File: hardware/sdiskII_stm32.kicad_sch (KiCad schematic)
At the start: 17 parts, among them J1 PWR, J2 APPLE_SDISKII, J3 Conn_01x06, J4 UART, J5 Conn_01x04, J6 STLINK, U2 MicroSD_SDIO, U8 DM-OLED096-636

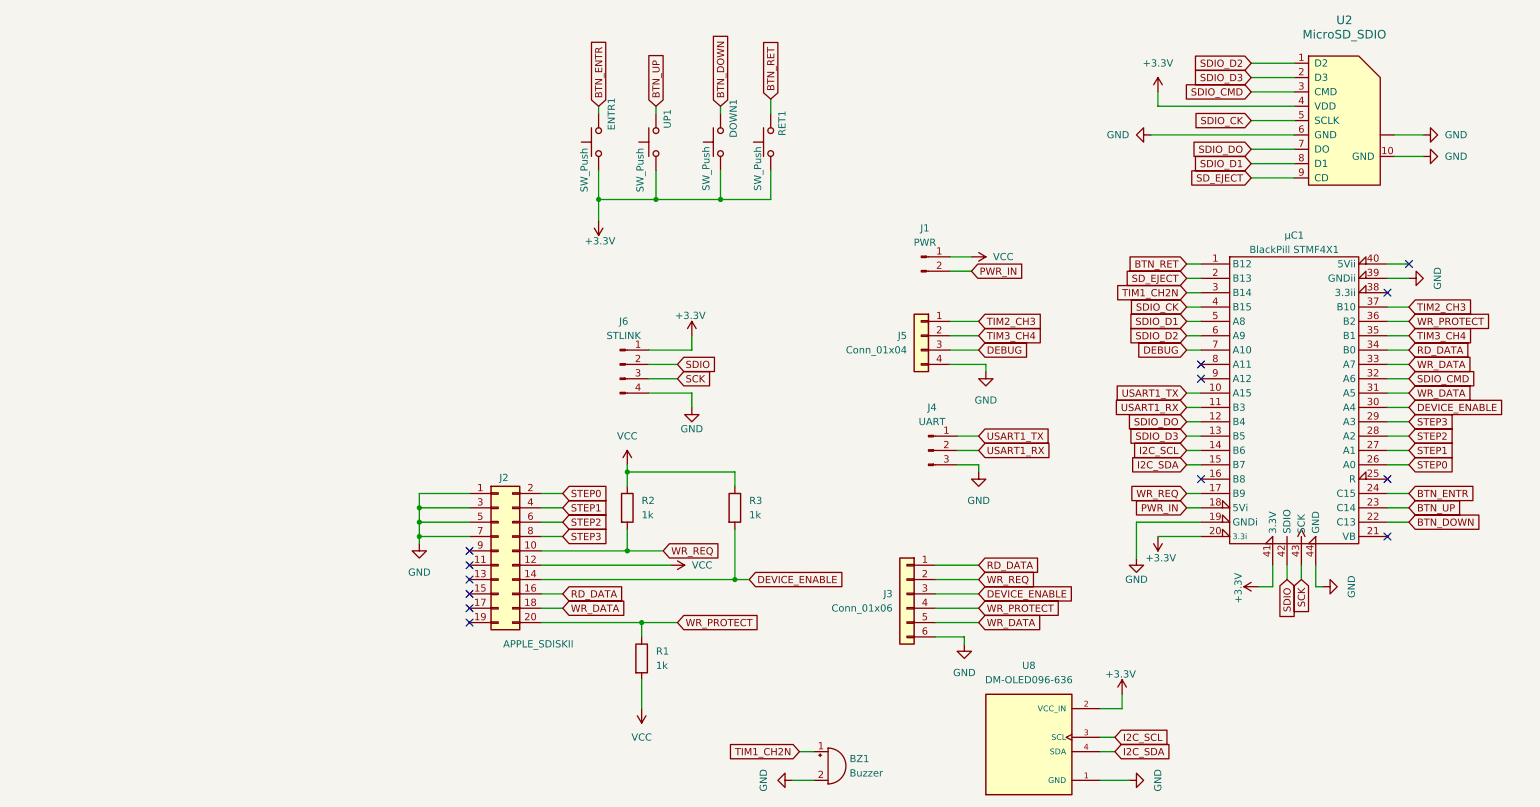
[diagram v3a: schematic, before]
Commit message: v0.79 Smartport HD working
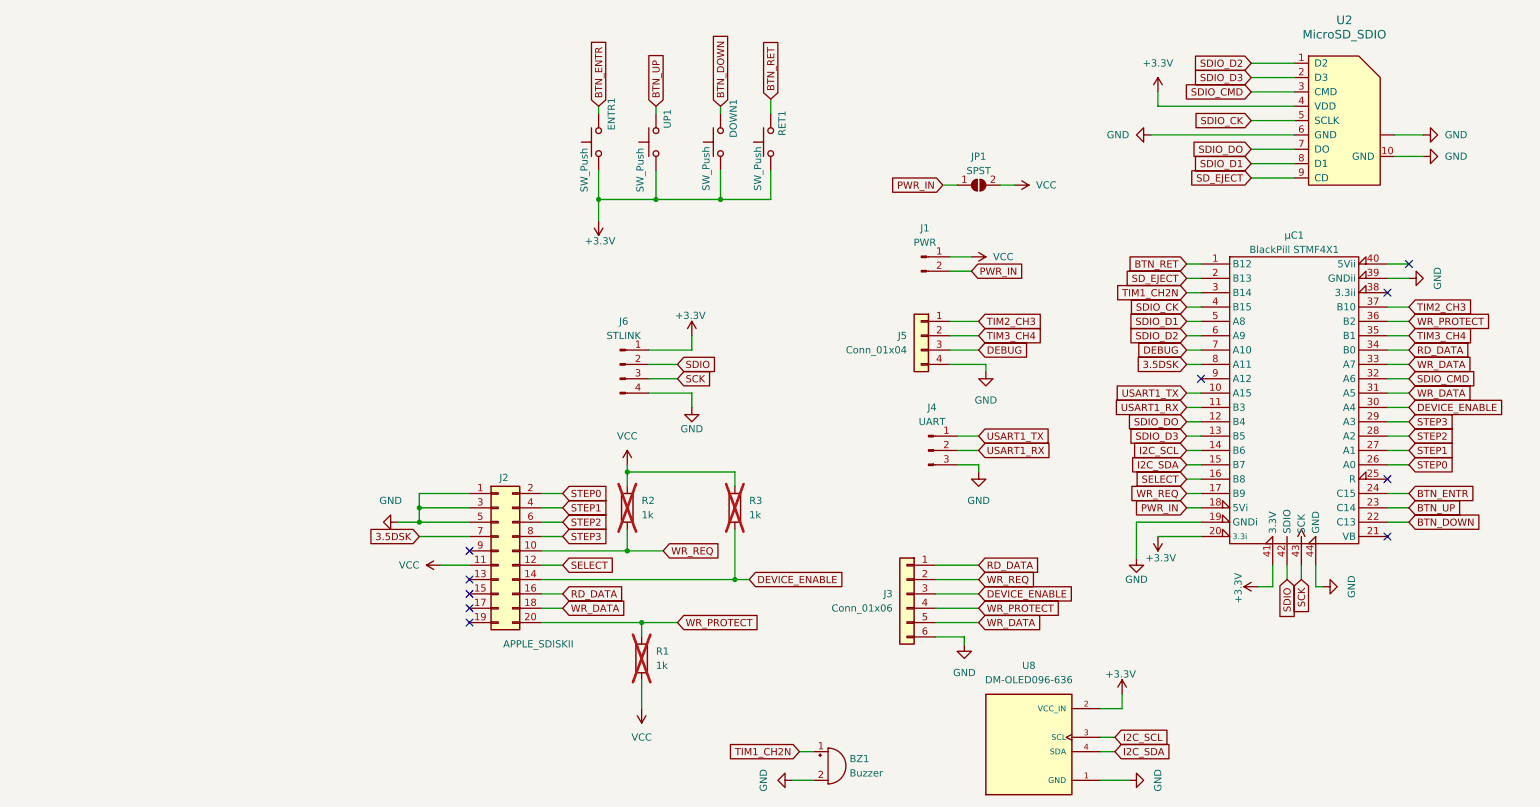
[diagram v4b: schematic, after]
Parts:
- added JP1: SPST, Jumper:SolderJumper-2_P1.3mm_Open_RoundedPad1.0x1.5mm, symbol Jumper:SolderJumper_2_Open
- R1, R2, R3: now not fitted
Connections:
- net GND: no longer J2.7 (Pin_7)
- net PWR_IN: now also JP1.1 (A)
- net VCC: now also J2.11 (Pin_11), JP1.2 (B); no longer J2.12 (Pin_12)
- net SELECT: now reaches μC1.16 (B8)
- net SELECT: now also J2.12 (Pin_12)
- net 3.5DSK: now reaches μC1.8 (A11)
- net 3.5DSK: now also J2.7 (Pin_7)
- no-connect marks 13 -> 10
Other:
- title: APPLE II DISK EM STM32F401 -> APPLE II DISK EM STM32F411
